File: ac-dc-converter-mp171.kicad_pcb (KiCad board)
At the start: 2 copper layers, 18 parts, among them J1 Conn_01x01, J2 Conn_01x01, J3 Conn_01x05, U1 MP171GJ

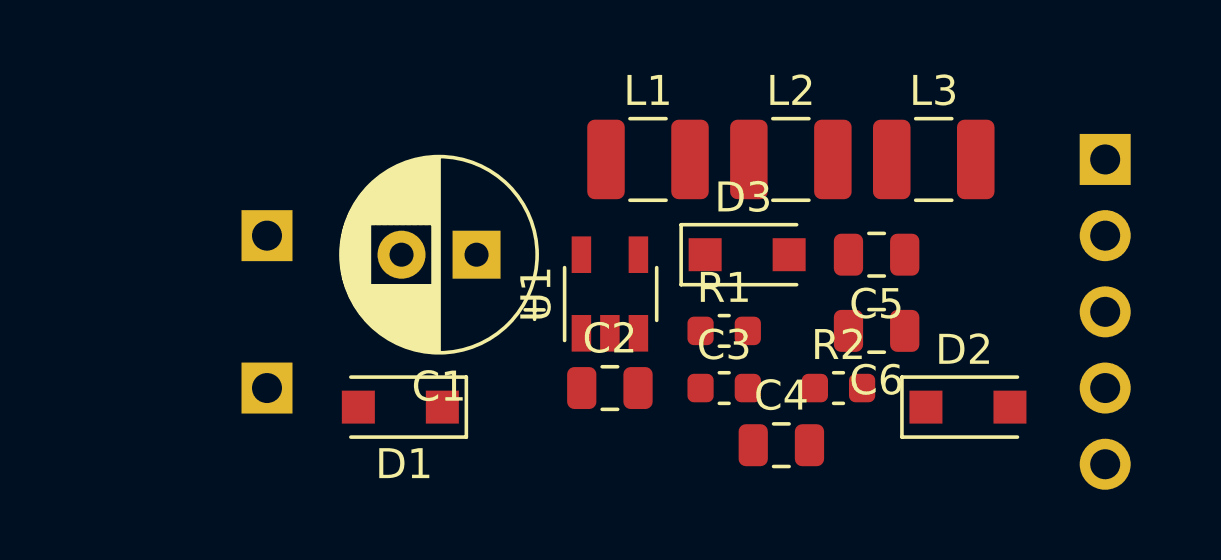
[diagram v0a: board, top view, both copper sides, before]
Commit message: completed so far. ready to order.
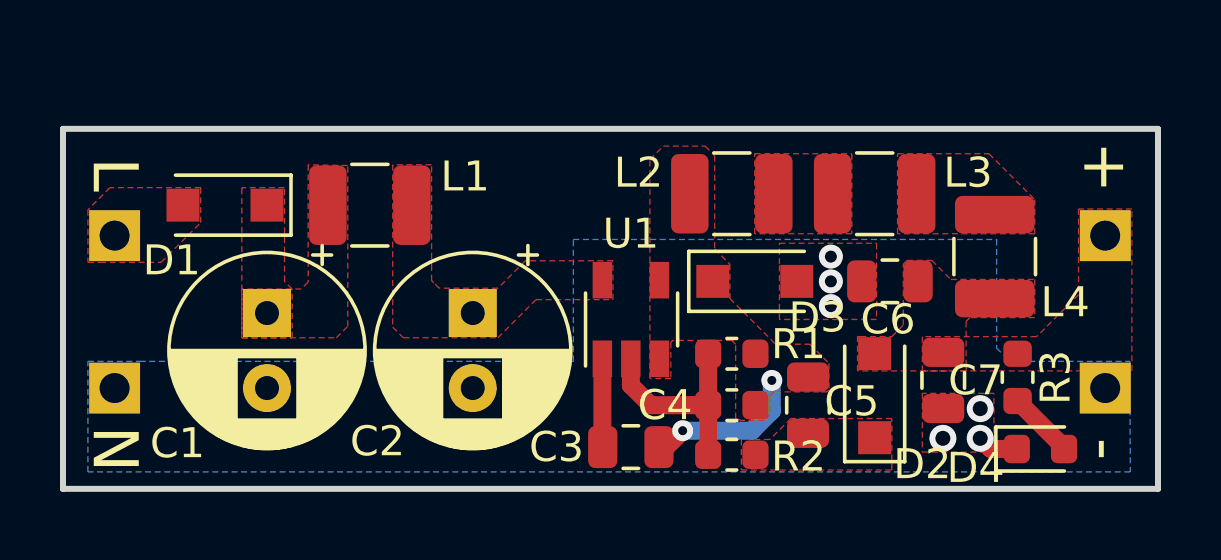
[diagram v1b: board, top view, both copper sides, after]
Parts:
- added C7: 10u_16V, Capacitor_SMD:C_0805_2012Metric, F.Cu at (136.8, 103.9)
- added D4: LED, LED_SMD:LED_0603_1608Metric, F.Cu at (140.1, 106.2)
- added J4: Conn_01x01, Connector_PinHeader_2.54mm:PinHeader_1x01_P2.54mm_Vertical, B.Cu at (142.2, 104.1)
- added L4: 330uH, Inductor_SMD:L_1210_3225Metric, F.Cu at (138.6, 99.8)
- added R3: 1K, Resistor_SMD:R_0603_1608Metric, F.Cu at (139.3, 103.8)
- C2: value 2.2u_25V -> 1u_400V; footprint Capacitor_SMD:C_0805_2012Metric -> Capacitor_THT:CP_Radial_D6.3mm_P2.50mm
- C3: value 1n_50V -> 2.2u_25V; footprint Capacitor_SMD:C_0603_1608Metric -> Capacitor_SMD:C_0805_2012Metric
- C4: value 1u_25V -> 1n_50V; footprint Capacitor_SMD:C_0805_2012Metric -> Capacitor_SMD:C_0603_1608Metric
- C5: value 10u_16V -> 1u_25V
- J3: value Conn_01x05 -> Conn_01x01; footprint Connector_PinHeader_2.54mm:PinHeader_1x05_P2.54mm_Vertical -> Connector_PinHeader_2.54mm:PinHeader_1x01_P2.54mm_Vertical
- moved L1 9.40 mm to (117.7, 98.0)
- moved D1 8.91 mm to (112.9, 98.0)
- moved C1 7.25 mm to (114.3, 101.6), turned to 270 degrees
- moved J1 7.18 mm to (109.2, 99.1)
- moved J2 7.18 mm to (109.2, 104.1)
- moved C5 5.51 mm to (132.3, 104.7), turned to 270 degrees
- moved C2 5.21 mm to (121.2, 101.6), turned to 270 degrees
- moved R2 4.19 mm to (129.8, 106.4)
- moved C3 3.68 mm to (126.4, 106.1)
- moved D2 3.13 mm to (134.6, 104.4), turned to 90 degrees
- moved J3 2.54 mm to (142.2, 99.1)
- moved L3 2.28 mm to (134.6, 97.7)
- moved L2 2.28 mm to (129.8, 97.7)
- moved C4 2.12 mm to (129.8, 104.7), turned to 180 degrees
- moved C6 1.71 mm to (135.1, 100.6)
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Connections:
- C1 pad 1: /DRAIN -> Net-(C1-Pad1)
- C2 pad 1: /VCC -> /DRAIN
- C2 pad 2: /SOURCE -> GND
- C3 pad 1: /SOURCE -> /VCC
- C3 pad 2: /FB -> /SOURCE
- C4 pad 2: Net-(C4-Pad2) -> /FB
- C5 pad 1: +5V1 -> /SOURCE
- C5 pad 2: GND -> Net-(C5-Pad2)
- C6 pad 1: +5V1 -> /+5V1
- D1 pad 1: /DRAIN -> Net-(C1-Pad1)
- D2 pad 1: Net-(C4-Pad2) -> Net-(C5-Pad2)
- D2 pad 2: +5V1 -> /+5V1
- J3 pad 1: +5V1 -> /+5V1
- L1 pad 1: /SOURCE -> Net-(C1-Pad1)
- L1 pad 2: Net-(L1-Pad2) -> /DRAIN
- L2 pad 1: Net-(L1-Pad2) -> /SOURCE
- L3 pad 2: +5V1 -> Net-(L3-Pad2)
- R2 pad 2: Net-(C4-Pad2) -> Net-(C5-Pad2)
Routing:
- net /FB: track 0.00 -> 7.10 mm
- net /SOURCE: track 0.00 -> 5.28 mm, vias 0 -> 2
- net /VCC: track 0.00 -> 2.95 mm
- net Net-(D4-Pad2): track 0.00 -> 2.24 mm
- net GND: track 0.00 -> 1.37 mm, vias 0 -> 6
- added copper zone on F.Cu, net /+5V1
- added copper zone on F.Cu, net /DRAIN
- added copper zone on F.Cu, net /L
- added copper zone on F.Cu, net /SOURCE
- added copper zone on B.Cu, net GND
- added copper zone on F.Cu, net GND
- added copper zone on F.Cu, net Net-(C1-Pad1)
- added copper zone on F.Cu, net Net-(C5-Pad2)
- added copper zone on F.Cu, net Net-(L2-Pad2)
- added copper zone on F.Cu, net Net-(L3-Pad2)
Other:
- board outline added: 36.5 x 12 mm
- board text added: "+"
- board text added: "-"
- board text added: "AC-DC Converter MP171 ©Projektanker"
- board text added: "L"
- board text added: "N"
